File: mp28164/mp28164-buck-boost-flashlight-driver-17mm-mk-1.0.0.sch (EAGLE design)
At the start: 20 parts, among them J1 AVR_SPI_PRG_6SMD-1.27MM, U1 MPS28164, U2 ATTINY25-20MU, U4 V_REG_ENTLV700

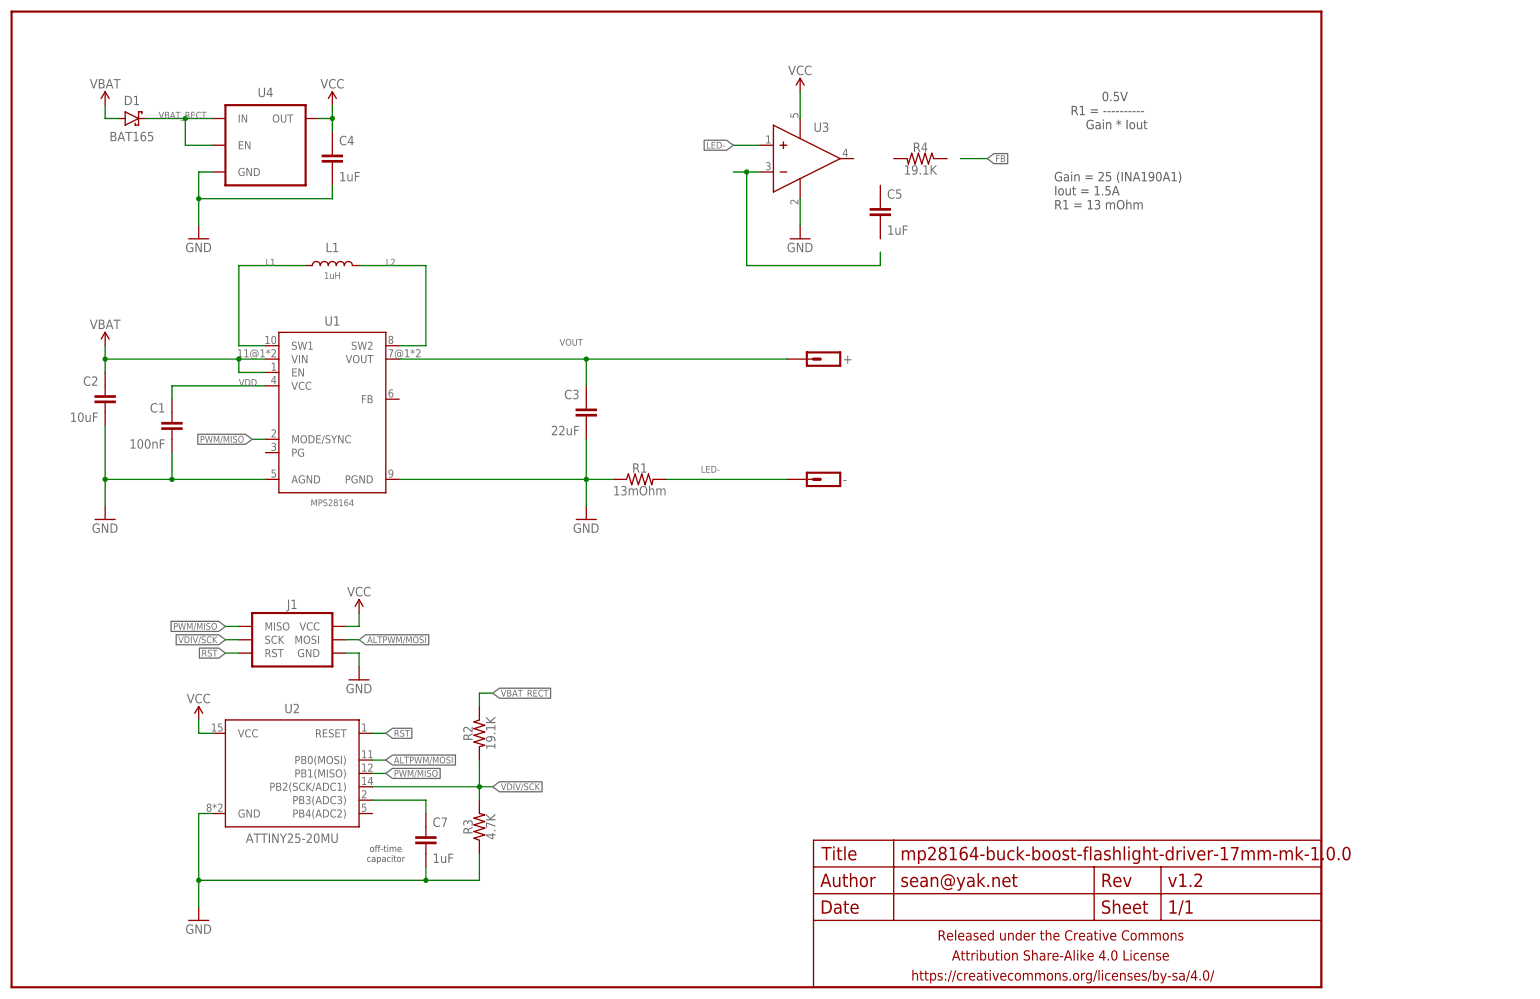
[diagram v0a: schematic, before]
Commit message: whole bunch of crap in here
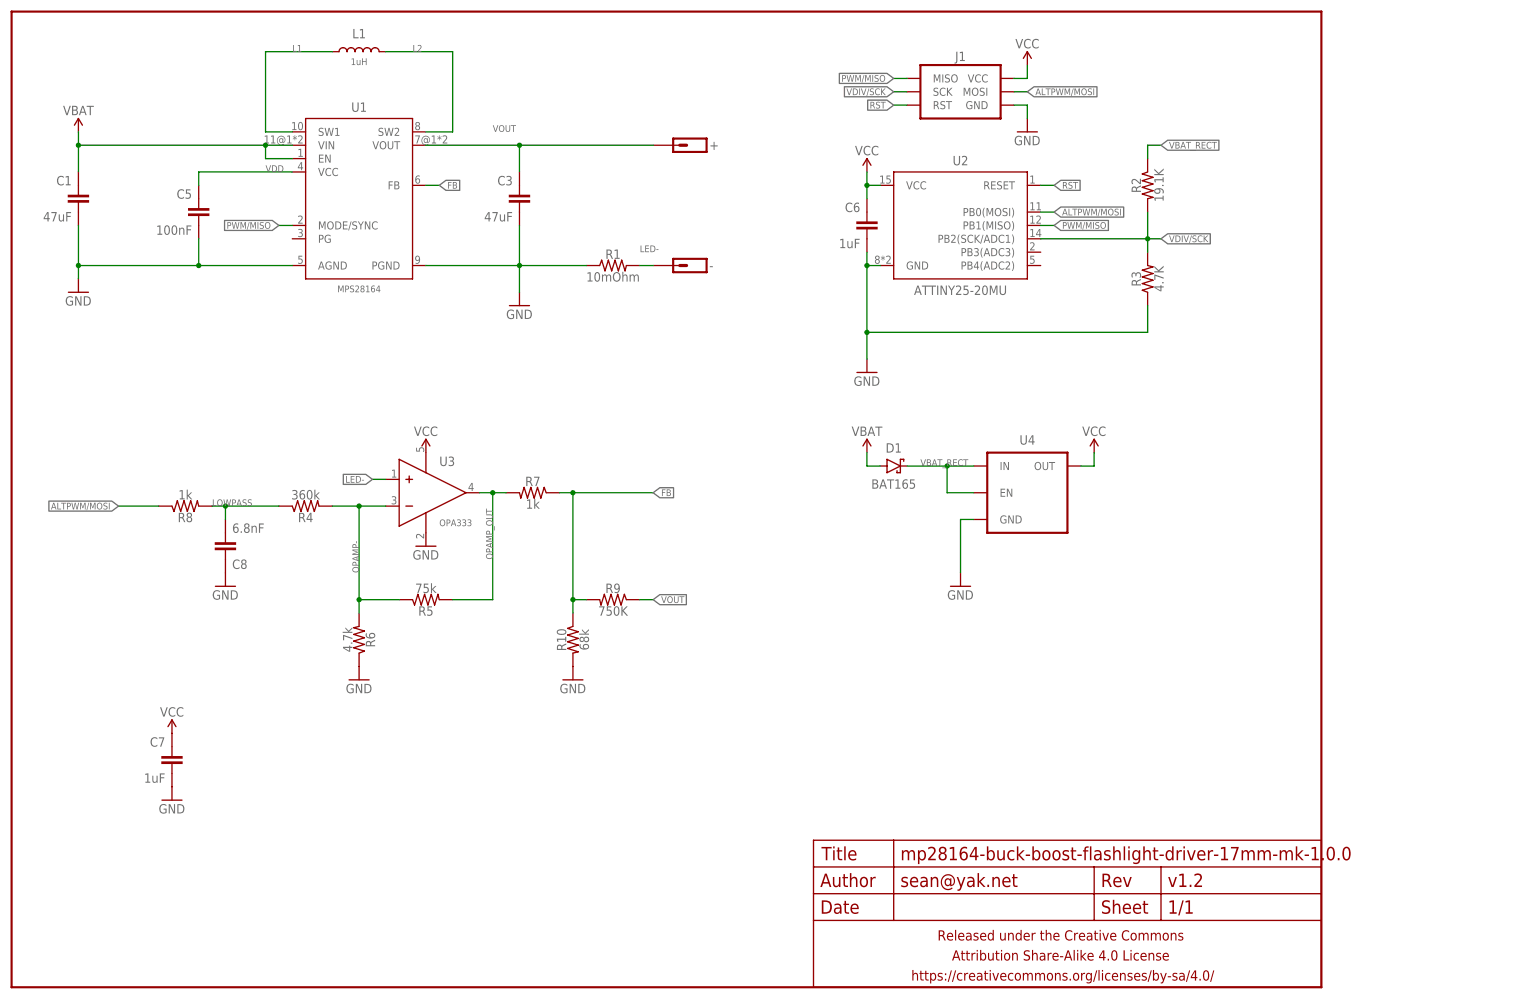
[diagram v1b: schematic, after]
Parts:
- removed C2: 10uF, a_parts:CAPACITOR-CERAMICC0805-TIGHTER
- removed C4: 1uF, a_parts:CAPACITOR-CERAMICC0402
- added C6: 1uF, a_parts:CAPACITOR-CERAMICC0402
- added C8: 6.8nF, a_parts:CAPACITOR-CERAMICC0402
- added R10: 68k, a_parts:RESISTORR0402
- added R5: 75k, a_parts:RESISTORR0402
- added R6: 4.7k, a_parts:RESISTORR0402
- added R7, R8: 1k, a_parts:RESISTORR0402
- added R9: 750K, a_parts:RESISTORR0402
- +, -: value M01PTH-1MM-CIR-NS -> M01SMD-1.6MMX3.2MM-NS; device a_parts:M01PTH-1MM-CIR-NS -> a_parts:M01SMD-1.6MMX3.2MM-NS
- C1: value 100nF -> 47uF; device a_parts:CAPACITOR-CERAMICC0402 -> a_parts:CAPACITOR-CERAMICC1206
- C3: value 22uF -> 47uF; device a_parts:CAPACITOR-CERAMICC0805-TIGHTER -> a_parts:CAPACITOR-CERAMICC1206
- C5: value 1uF -> 100nF
- L1: device a_parts:INDUCTORXAR7030 -> a_parts:INDUCTORXAL7070
- R1: value 13mOhm -> 10mOhm
- R4: value 19.1K -> 360k
- U3: value (none) -> OPA333
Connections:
- removed net N$1: U3.IN-
- removed net N$5: C7.1, U2.PB3(ADC3)
- new net FB: R10.1, R7.1, R9.2, U1.FB
- new net LOWPASS: C8.2, R4.1, R8.2
- new net OPAMP-: R4.2, R5.1, R6.2, U3.IN-
- new net OPAMP_OUT: R5.2, R7.2, U3.OUT
- net ALTPWM/MOSI: now also R8.1
- net GND: now also C5.2, C6.2, C8.1, R10.2, R6.1; no longer C2.2, C4.2
- net VBAT: now also C1.1; no longer C2.1
- net VCC: now also C6.1, C7.1; no longer C4.1
- net VDD: now also C5.1; no longer C1.1
- net VOUT: now also R9.1
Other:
- note added: "Current Sense Multiplier"
- note added: "Fallback Voltage"
- note added: "Low-pass Filter"
- note removed: "0.5V R1 = ---------- Gain * Iout"
- note removed: "Gain = 25 (INA190A1) Iout = 1.5A R1 = 13 mOhm"
- note removed: "off-time capacitor"
- moved on the sheet: +, -, C1, C3, C5, C7, D1, J1, L1, R1, R2, R3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
